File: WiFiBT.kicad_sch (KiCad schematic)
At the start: 1 part, among them U2 ESP32-D0WD-V3

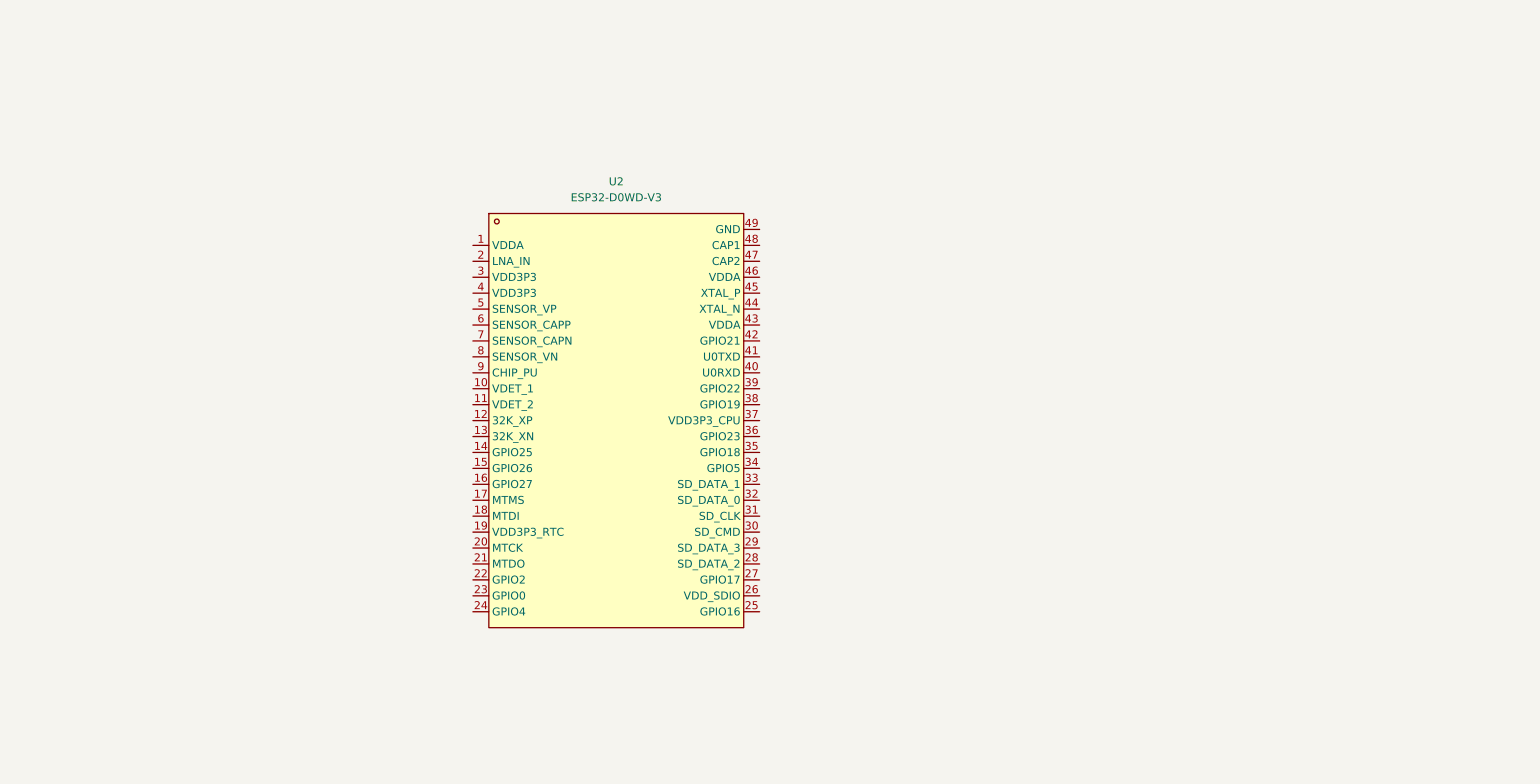
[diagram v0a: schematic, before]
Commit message: before switching to ESP32 module
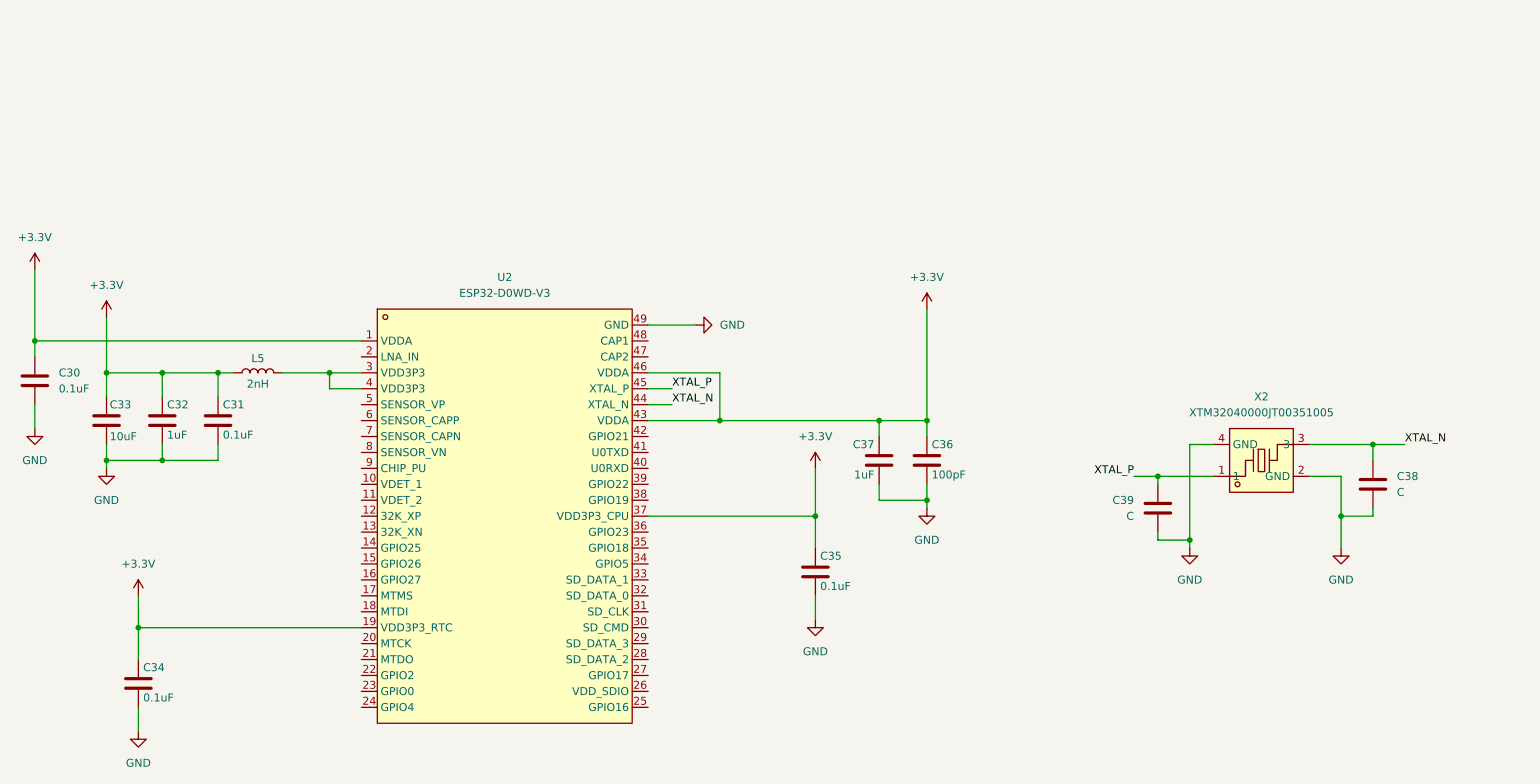
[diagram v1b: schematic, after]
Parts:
- added C30, C31, C34, C35: 0.1uF, symbol Device:C
- added C32, C37: 1uF, symbol Device:C
- added C33: 10uF, symbol Device:C
- added C36: 100pF, symbol Device:C
- added C38, C39: C, symbol Device:C
- added L5: 2nH, symbol Device:L
- added X2: XTM32040000JT00351005, easyeda2kicad:CRYSTAL-SMD_4P-L3.2-W2.5-BL, symbol easyeda2kicad:XTM32040000JT00351005
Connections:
- net +3.3V: now reaches U2.1 (VDDA)
- net +3.3V: now also U2.19 (VDD3P3_RTC), U2.37 (VDD3P3_CPU), U2.43 (VDDA), U2.46 (VDDA), C30.1, C31.1, C32.1, C33.1, C34.1, C35.1, C36.1, C37.1, L5.1
- net at U2.3 (VDD3P3): now also U2.4 (VDD3P3), L5.2
- net XTAL_N: now reaches U2.44 (XTAL_N)
- net XTAL_N: now also C38.1, X2.3
- net XTAL_P: now reaches U2.45 (XTAL_P)
- net XTAL_P: now also C39.1, X2.1
- net GND: now reaches U2.49 (GND)
- net GND: now also C30.2, C31.2, C32.2, C33.2, C34.2, C35.2, C36.2, C37.2, C38.2, C39.2, X2.2 (GND), X2.4 (GND)
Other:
- moved on the sheet: U2

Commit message: start of adding esp32 module
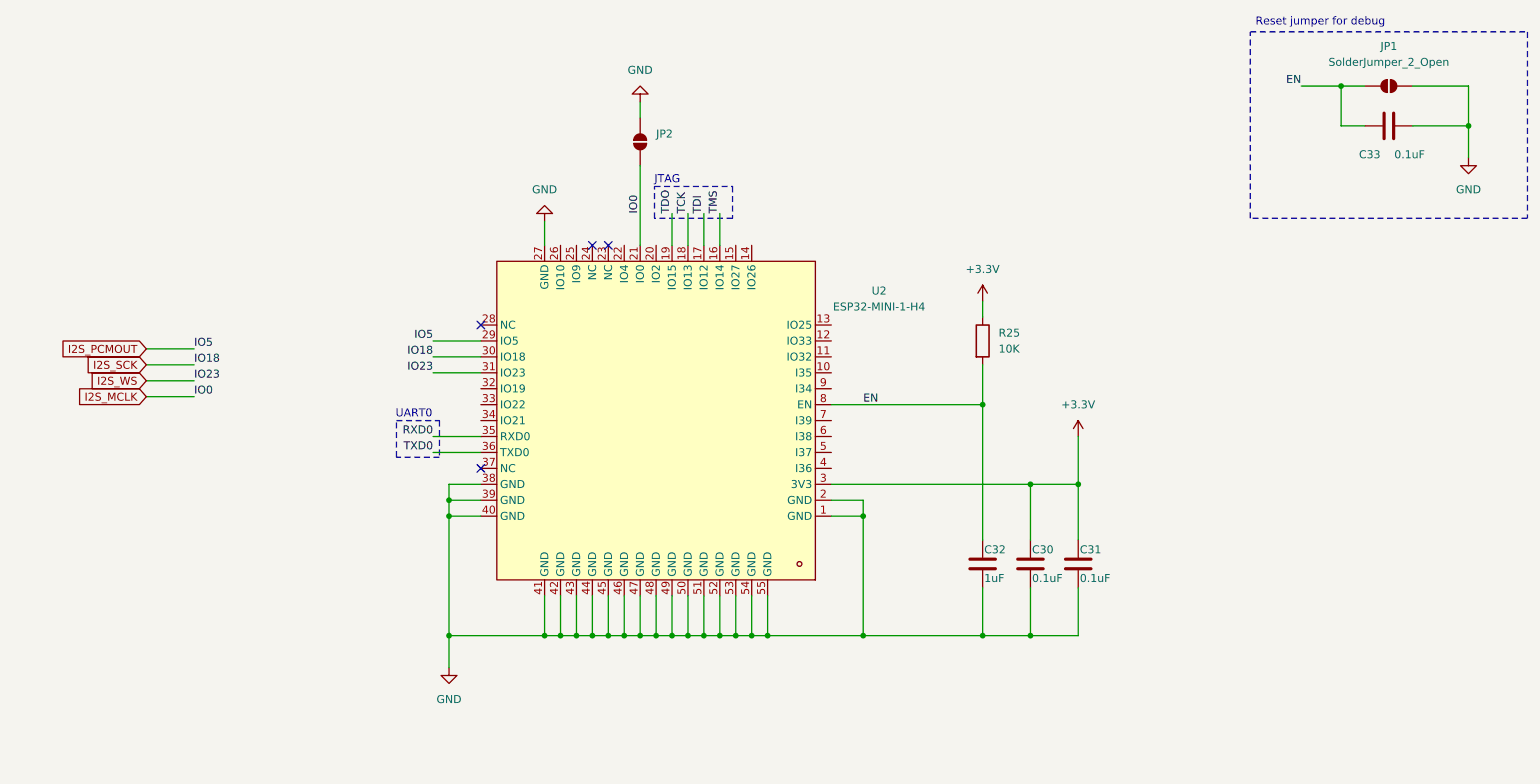
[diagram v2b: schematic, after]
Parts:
- removed C34, C35: 0.1uF, symbol Device:C
- removed C36: 100pF, symbol Device:C
- removed C37: 1uF, symbol Device:C
- removed C38, C39: C, symbol Device:C
- removed L5: 2nH, symbol Device:L
- removed U2: ESP32-D0WD-V3, easyeda2kicad:QFN-48_L5.0-W5.0-P0.35-BL-EP3.7, symbol easyeda2kicad:ESP32-D0WD-V3
- removed X2: XTM32040000JT00351005, easyeda2kicad:CRYSTAL-SMD_4P-L3.2-W2.5-BL, symbol easyeda2kicad:XTM32040000JT00351005
- added JP1, JP2: SolderJumper_2_Open, symbol Jumper:SolderJumper_2_Open
- added R25: 10K, symbol Device:R
- added U2: ESP32-MINI-1-H4, easyeda2kicad:WIFI-SMD_ESP32-MINI-1, symbol easyeda2kicad:ESP32-MINI-1-H4
- C33: value 10uF -> 0.1uF
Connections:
- net +3.3V: now also R25.1, U2.3 (3V3); no longer C32.1, C33.1
- net GND: now also JP1.2 (B), JP2.2 (B), U2.1 (GND), U2.2 (GND), U2.27 (GND), U2.38 (GND), U2.39 (GND), U2.40 (GND), U2.41 (GND), U2.42 (GND), U2.43 (GND), U2.44 (GND), U2.45 (GND), U2.46 (GND), U2.47 (GND), U2.48 (GND), U2.49 (GND), U2.50 (GND), U2.51 (GND), U2.52 (GND), U2.53 (GND), U2.54 (GND), U2.55 (GND)
- new net EN: C32.1, C33.1, JP1.1 (A), R25.2, U2.8 (EN)
- new net I2S_MCLK: JP2.1 (A), U2.21 (IO0)
- new net I2S_PCMOUT: U2.29 (IO5)
- new net I2S_SCK: U2.30 (IO18)
- new net I2S_WS: U2.31 (IO23)
- new net RXD0: U2.35 (RXD0)
- new net TCK: U2.18 (IO13)
- new net TDI: U2.17 (IO12)
- new net TDO: U2.19 (IO15)
- new net TMS: U2.16 (IO14)
- new net TXD0: U2.36 (TXD0)
- no-connect marks 0 -> 4
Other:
- note added: "JTAG"
- note added: "Reset jumper for debug"
- note added: "UART0"
